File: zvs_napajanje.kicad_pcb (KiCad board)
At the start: 2 copper layers, 75.5 x 98.5 mm, 20 parts, among them J1 ulaz, J2 Conn_01x01_Female, J3 Conn_01x01_Female, J4 Conn_01x01_Female, Q1 IRFP250, Q2 IRFP250

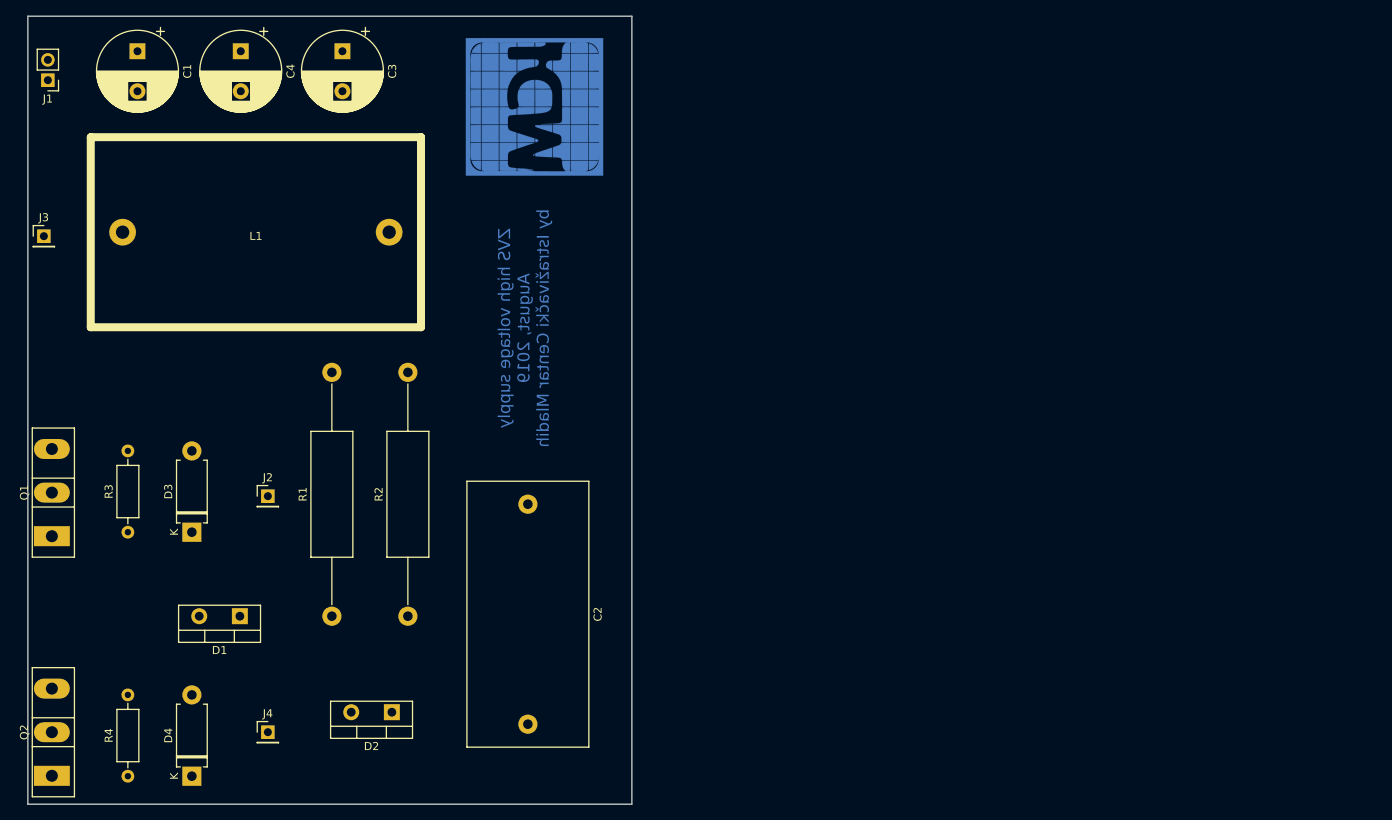
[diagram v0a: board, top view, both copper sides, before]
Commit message: almost almost over
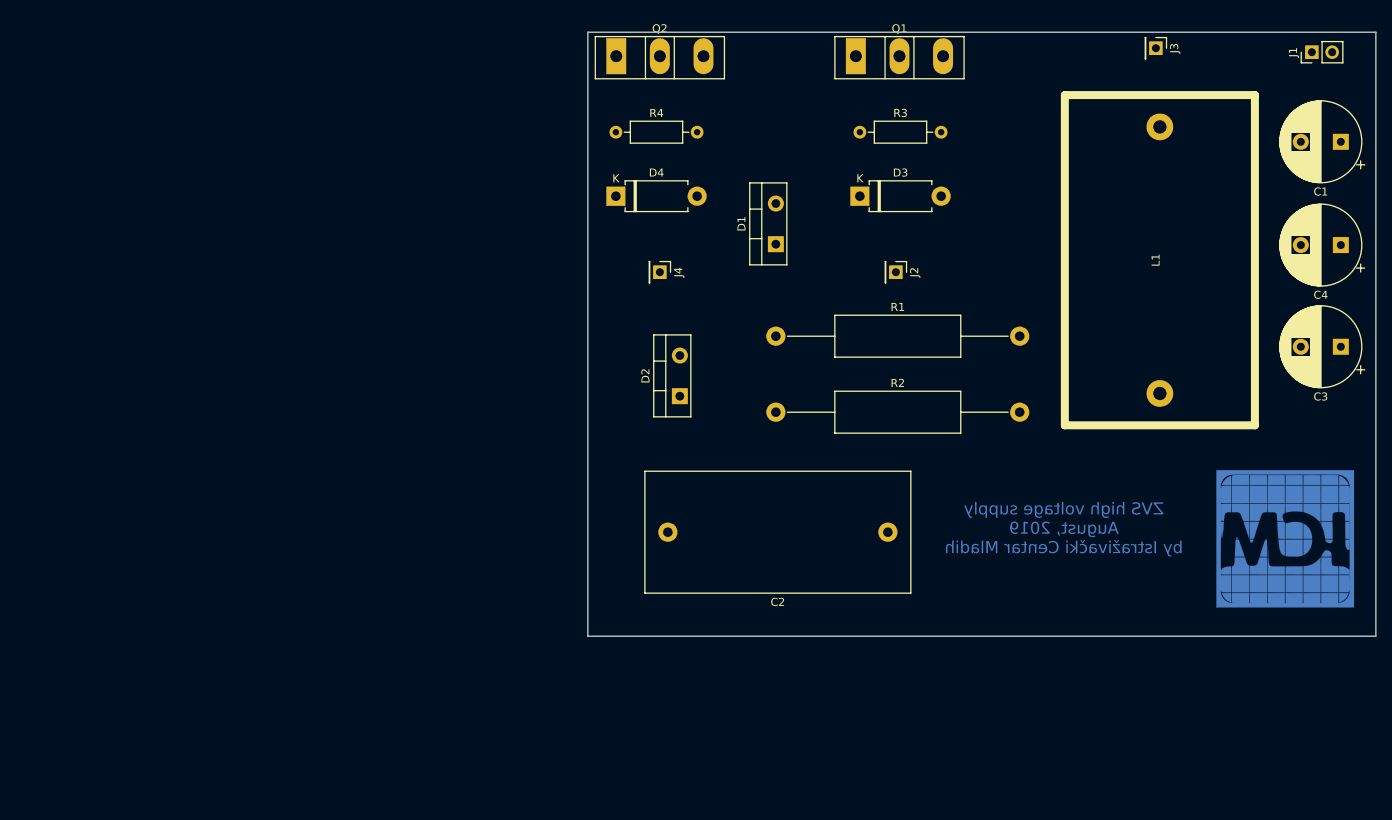
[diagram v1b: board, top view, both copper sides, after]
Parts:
- moved J1 158.0 mm to (192.5, 63.5), turned to 90 degrees
- moved C1 150.8 mm to (196.1, 74.7), turned to 180 degrees
- moved J3 141.0 mm to (173.0, 63.0), turned to 270 degrees
- moved C4 139.6 mm to (196.1, 87.6), turned to 180 degrees
- moved C3 130.2 mm to (196.1, 100.3), turned to 180 degrees
- moved Q1 117.0 mm to (135.5, 64.0), turned to 0 degrees
- moved Q2 114.3 mm to (105.5, 64.0), turned to 0 degrees
- moved L1 113.1 mm to (173.5, 89.5), turned to 270 degrees
- moved G*** 107.3 mm to (188.5, 124.5), turned to 0 degrees
- moved R3 104.3 mm to (136.0, 73.5), turned to 0 degrees
- moved R4 101.0 mm to (105.5, 73.5), turned to 0 degrees
- moved D3 93.5 mm to (136.0, 81.5), turned to 0 degrees
- moved D4 89.8 mm to (105.5, 81.5), turned to 0 degrees
- moved J2 83.3 mm to (140.5, 91.0), turned to 270 degrees
- moved D1 81.6 mm to (125.5, 87.5), turned to 90 degrees
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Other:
- board size 75.5 x 98.5 mm -> 98.5 x 75.5 mm
